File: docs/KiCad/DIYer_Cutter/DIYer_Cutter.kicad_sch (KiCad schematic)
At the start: 68 parts, among them M1 Stepper_Motor_bipolar, M2 Motor_Servo, Q1 2N2219, SW1 SW_Push, U1 micro:bit, U2 MCP23008-xP, U3 MCP23008-xP, U4 keypad_3x4_matrix, U5 MCP23008-xP, U6 easy_stepper_driver, U7 74HCT125, U8 74HC245

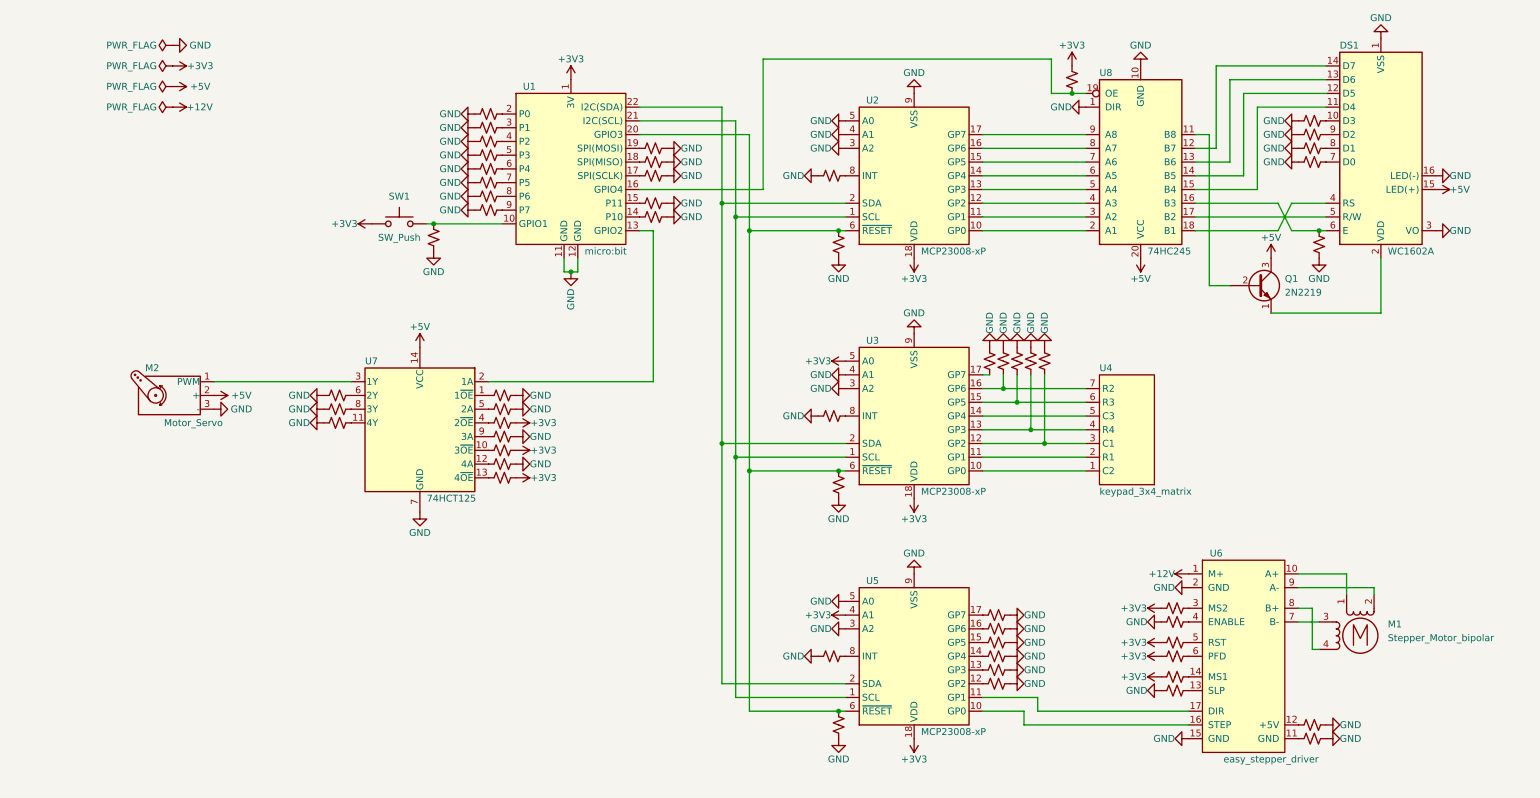
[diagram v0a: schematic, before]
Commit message: Probably working devcontainers config
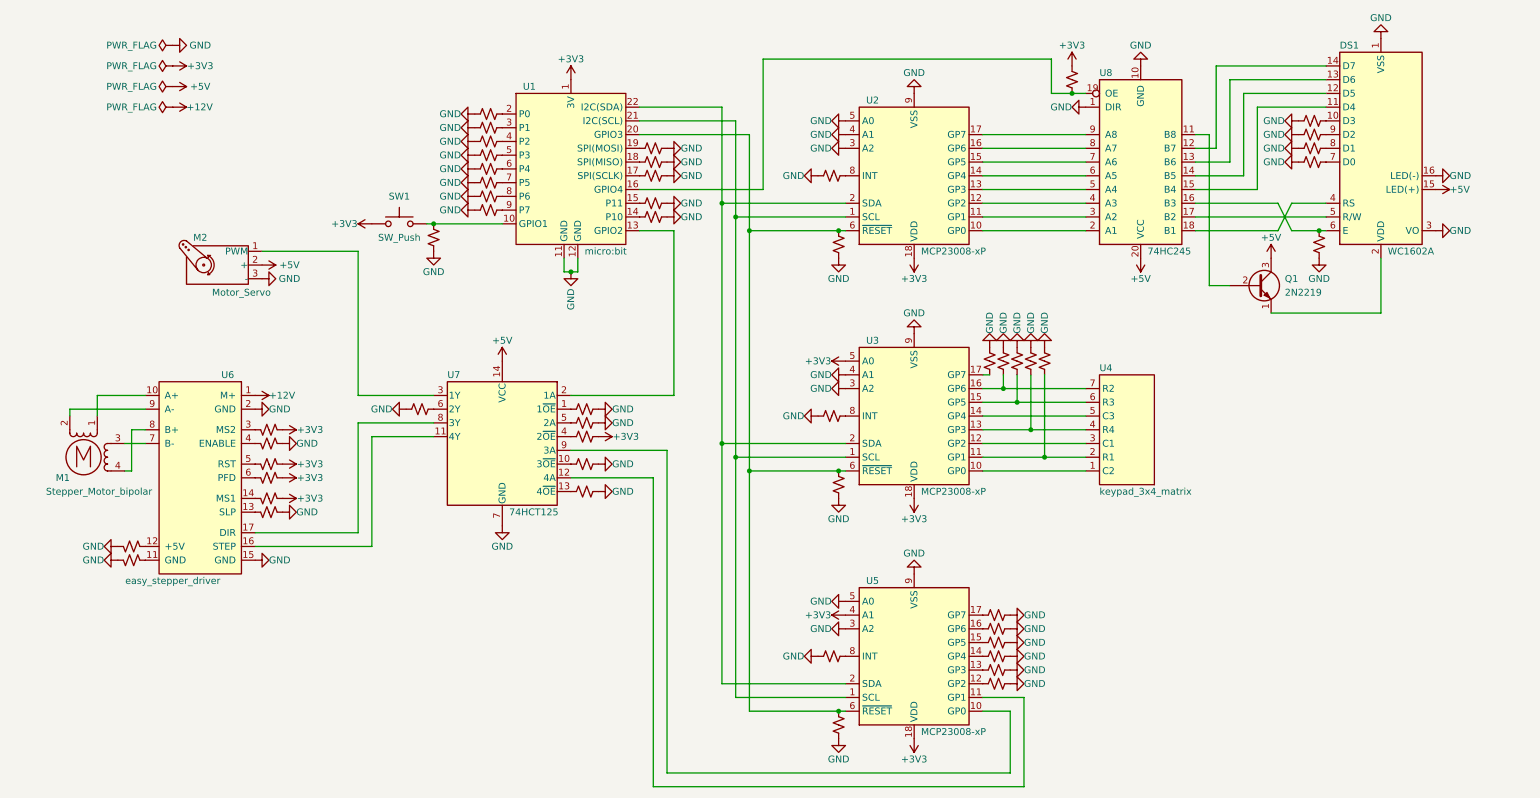
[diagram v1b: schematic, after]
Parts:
- removed R22, R48, R50, R58: R_Small_US, symbol Device:R_Small_US
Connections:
- net +3V3: no longer R49.1, R51.1
- net GND: now also R21.2, R49.1, R51.1; no longer R21.1
- net at U7.9 (3A): now also U5.10 (GP0)
- net at U6.16 (STEP): now also U7.11 (4Y); no longer U5.10 (GP0)
- net at U6.17 (DIR): now also U7.8 (3Y); no longer U5.11 (GP1)
- net at U7.12 (4A): now also U5.11 (GP1)
- net at U3.11 (GP1), U4.2 (R1): now also R52.2
- net at U3.12 (GP2), U4.3 (C1): no longer R52.2
- net at U5.8 (INT): now also R21.1
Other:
- moved on the sheet: M1, M2, U6, U7
